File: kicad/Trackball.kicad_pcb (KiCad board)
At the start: 2 copper layers, 44 x 44 mm, 40 parts, among them J1 Conn_01x04, J2 Conn_02x10_Odd_Even, SW1 SW_Push, SW2 SW_Push, U1 TCR2EF19, U2 PMW3360, U3 RP2040, U4 TLV73333PDBV, U5 W25Q128JVS, Y1 Crystal_GND24

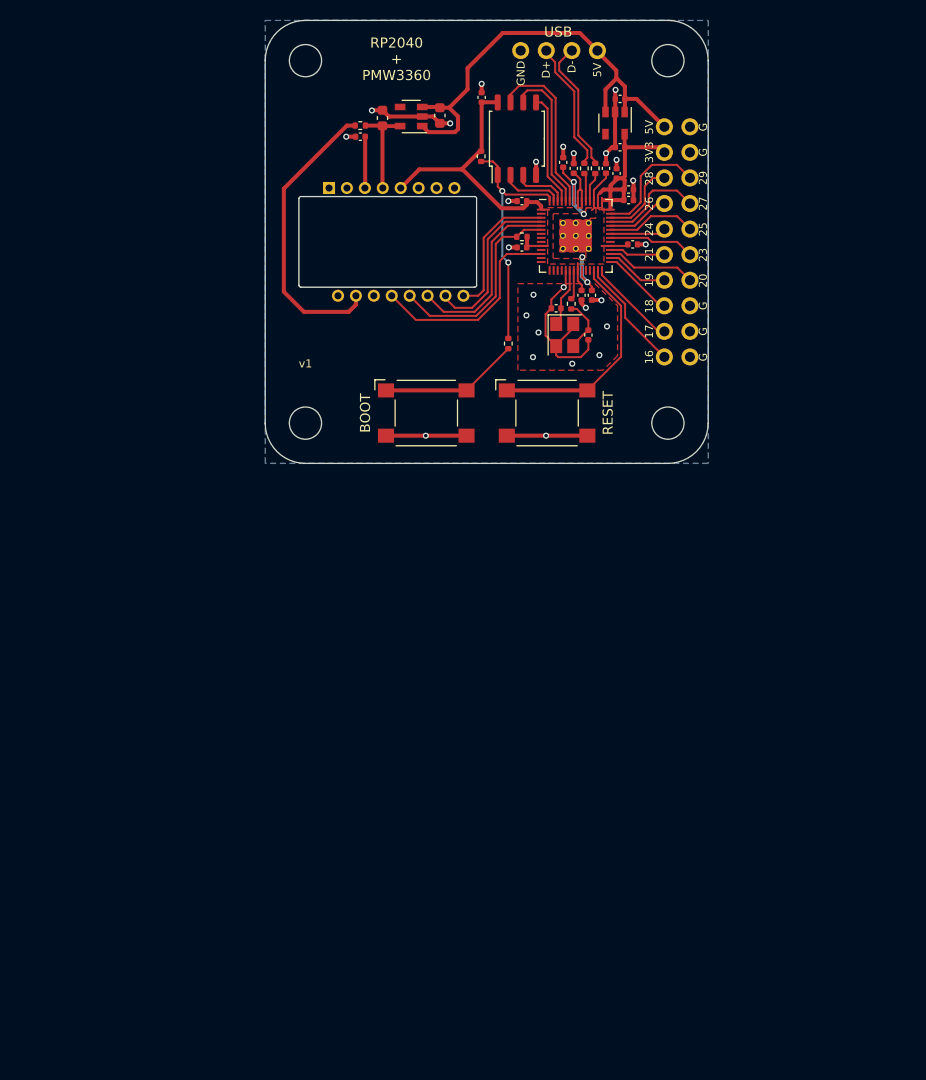
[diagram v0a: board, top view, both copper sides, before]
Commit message: x
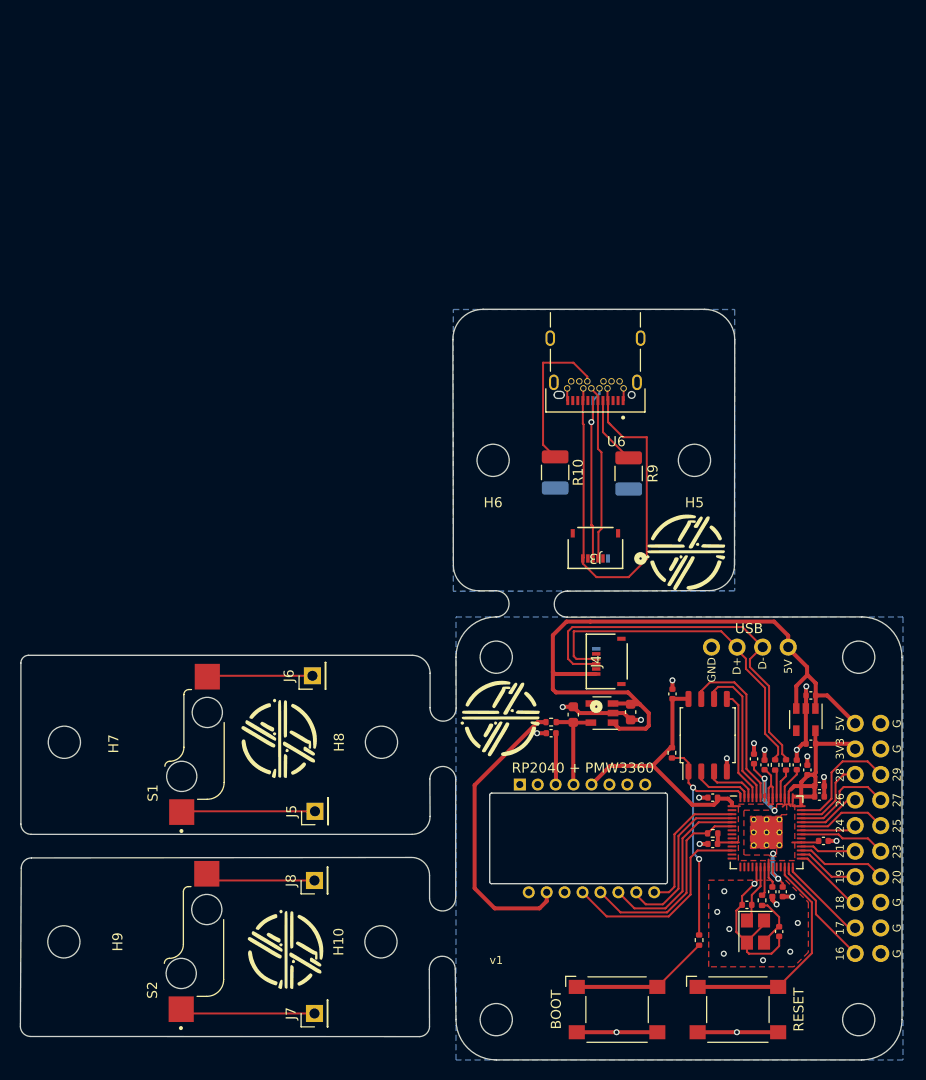
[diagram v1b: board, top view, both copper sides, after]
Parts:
- added G***: LOGO, LOGO, F.Cu at (102.8, 118.4)
- added G***: LOGO, LOGO, F.Cu at (102.2, 97.4)
- added G***: LOGO, LOGO, F.Cu at (142.9, 79.0)
- added G***: LOGO, LOGO, F.Cu at (124.4, 95.5)
- added G***: LOGO, LOGO, B.Cu at (124.4, 95.5)
- added G***: LOGO, LOGO, B.Cu at (142.9, 79.0)
- added G***: LOGO, LOGO, B.Cu at (102.8, 97.4)
- added G***: LOGO, LOGO, B.Cu at (102.8, 118.4)
- added H10: MountingHole, MountingHole:MountingHole_3.2mm_M3, F.Cu at (112.5, 117.5)
- added H5: MountingHole, MountingHole:MountingHole_3.2mm_M3, F.Cu at (143.6, 69.7)
- added H6: MountingHole, MountingHole:MountingHole_3.2mm_M3, F.Cu at (123.6, 69.7)
- added H7: MountingHole, MountingHole:MountingHole_3.2mm_M3, F.Cu at (81.1, 97.7)
- added H8: MountingHole, MountingHole:MountingHole_3.2mm_M3, F.Cu at (112.5, 97.7)
- added H9: MountingHole, MountingHole:MountingHole_3.2mm_M3, F.Cu at (81.0, 117.5)
- added J3: FH34SRJ-6S-0.5SH50, footprints:CONN6x1_FH34SRJ-6S-0.5SH50_HIR, F.Cu at (133.8, 78.4)
- added J4: FH34SRJ-6S-0.5SH50, footprints:CONN6x1_FH34SRJ-6S-0.5SH50_HIR, F.Cu at (134.9, 89.7)
- added J5: Conn_01x01, Connector_PinHeader_2.54mm:PinHeader_1x01_P2.54mm_Vertical, F.Cu at (105.9, 104.6)
- added J6: Conn_01x01, Connector_PinHeader_2.54mm:PinHeader_1x01_P2.54mm_Vertical, F.Cu at (105.7, 91.1)
- added J7: Conn_01x01, Connector_PinHeader_2.54mm:PinHeader_1x01_P2.54mm_Vertical, F.Cu at (105.9, 124.6)
- added J8: Conn_01x01, Connector_PinHeader_2.54mm:PinHeader_1x01_P2.54mm_Vertical, F.Cu at (105.9, 111.4)
- added R10: 5.1k, Resistor_SMD:R_1210_3225Metric_Pad1.30x2.65mm_HandSolder, F.Cu at (129.8, 70.9)
- added R9: 5.1k, Resistor_SMD:R_1210_3225Metric_Pad1.30x2.65mm_HandSolder, F.Cu at (137.1, 71.0)
- added S1: PG151101S11, Kailk SMD socket PG151101S11:SW_PG151101S11, F.Cu at (94.0, 97.9)
- added S2: PG151101S11, Kailk SMD socket PG151101S11:SW_PG151101S11, F.Cu at (93.9, 117.5)
- added U6: TYPE-C-31-M-14, TypeC:AMPHENOL_GSB3CA11310DSHR, F.Cu at (133.8, 63.2)
- moved U5 62.2 mm to (150.8, 106.7)
- moved C10 62.2 mm to (153.8, 100.0)
- moved C11 62.2 mm to (152.4, 112.5)
- moved C17 62.2 mm to (151.4, 112.5)
- moved C19 62.2 mm to (156.1, 102.0)
- moved C2 62.2 mm to (152.1, 116.5)
- moved C4 62.2 mm to (129.4, 96.8)
- moved C6 62.2 mm to (137.3, 94.7)
- moved H1 62.2 mm to (124.0, 89.2)
- moved H2 62.2 mm to (124.0, 125.2)
- moved R3 62.2 mm to (141.4, 98.8)
- moved R4 62.2 mm to (129.4, 95.7)
- moved R6 62.2 mm to (151.7, 100.0)
- moved C18 62.2 mm to (156.1, 103.1)
- moved C7 62.2 mm to (141.4, 92.9)
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- renumbered C18 to C1, C13 to C10, C2 to C11, C3 to C12, C4 to C13, C5 to C14, C6 to C15, C10 to C16, C7 to C17, C8 to C18, C9 to C19, C19 to C2, C15 to C3, C14 to C4, C16 to C5, C11 to C6, C17 to C7, C12 to C8, C1 to C9, J2 to J1, J1 to J2, R7 to R1, R6 to R2, R5 to R3, R1 to R4, R2 to R5, R3 to R6, R4 to R7, SW2 to SW1, SW1 to SW2, U4 to U1, U5 to U3, U1 to U4, U3 to U5
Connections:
- net GND renamed GND-USB
- U1 pad 4: Net-(U4-Pad4) -> unconnected-(U1-NC-Pad4)
- U2 pad 1: Net-(U2-Pad1) -> unconnected-(U2-NC-Pad1)
- U2 pad 14: Net-(U2-Pad14) -> unconnected-(U2-NC-Pad14)
- U2 pad 16: Net-(U2-Pad16) -> unconnected-(U2-NC-Pad16)
- U2 pad 2: Net-(U2-Pad2) -> unconnected-(U2-NC-Pad2)
- U2 pad 6: Net-(U2-Pad6) -> unconnected-(U2-NC-Pad6)
- U2 pad 7: Net-(U2-Pad7) -> unconnected-(U2-NRESET-Pad7)
- U4 pad 4: Net-(U1-Pad4) -> unconnected-(U4-NC-Pad4)
- U5 pad 11: Net-(U3-Pad11) -> unconnected-(U5-GPIO8-Pad11)
- U5 pad 13: Net-(U3-Pad13) -> unconnected-(U5-GPIO10-Pad13)
- U5 pad 14: Net-(U3-Pad14) -> unconnected-(U5-GPIO11-Pad14)
- U5 pad 15: Net-(U3-Pad15) -> unconnected-(U5-GPIO12-Pad15)
- U5 pad 16: Net-(U3-Pad16) -> unconnected-(U5-GPIO13-Pad16)
- U5 pad 17: Net-(U3-Pad17) -> unconnected-(U5-GPIO14-Pad17)
- U5 pad 18: Net-(U3-Pad18) -> unconnected-(U5-GPIO15-Pad18)
- U5 pad 2: Net-(U3-Pad2) -> unconnected-(U5-GPIO0-Pad2)
- U5 pad 24: Net-(U3-Pad24) -> unconnected-(U5-SWCLK-Pad24)
- U5 pad 25: Net-(U3-Pad25) -> unconnected-(U5-SWD-Pad25)
- U5 pad 34: Net-(U3-Pad34) -> unconnected-(U5-GPIO22-Pad34)
- U5 pad 7: Net-(U3-Pad7) -> unconnected-(U5-GPIO5-Pad7)
- U5 pad 8: Net-(U3-Pad8) -> unconnected-(U5-GPIO6-Pad8)
- U5 pad 9: Net-(U3-Pad9) -> unconnected-(U5-GPIO7-Pad9)
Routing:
- net +: track 0.00 -> 45.4 mm
- net D-: track 13.2 -> 39.3 mm
- net +5V: track 45.0 -> 70.0 mm
- net D+: track 13.0 -> 34.7 mm
- net DN: track 0.00 -> 19.6 mm, vias 0 -> 1
- net DP: track 0.00 -> 17.5 mm
- net Net-(R10-+): track 0.00 -> 15.4 mm
- net Net-(J7-Pin_1): track 0.00 -> 13.4 mm
- net Net-(J5-Pin_1): track 0.00 -> 13.3 mm
- net Net-(J8-Pin_1): track 0.00 -> 11.0 mm
- net Net-(J6-Pin_1): track 0.00 -> 10.5 mm
- net Net-(R9-+): track 0.00 -> 6.75 mm
- net GND-USB: track 61.8 -> 64.3 mm
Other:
- board size 44 x 44 mm -> 87.6 x 74.6 mm
- net class Default removed
- net class Power removed
- net class dPair removed
- board text added: "github.com/bigFin/rp2040-pmw3360"
- board text removed: "github.com/jfedor2/rp2040-pmw3360"
